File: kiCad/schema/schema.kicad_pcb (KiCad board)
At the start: 2 copper layers, 103.8 x 139.4 mm, 20 parts, among them J1 Conn_01x06_Pin, J11 Switch, J12 Conn_01x15_Pin, J13 Conn_01x15_Pin, J14 Conn_01x06_Pin, J3 M1 Right, J4 M2 Left, J5 Bat, J6 Buck, Q1 Q_Photo_NPN, Q2 Q_Photo_NPN, Q3 Q_Photo_NPN, Q4 Q_Photo_NPN

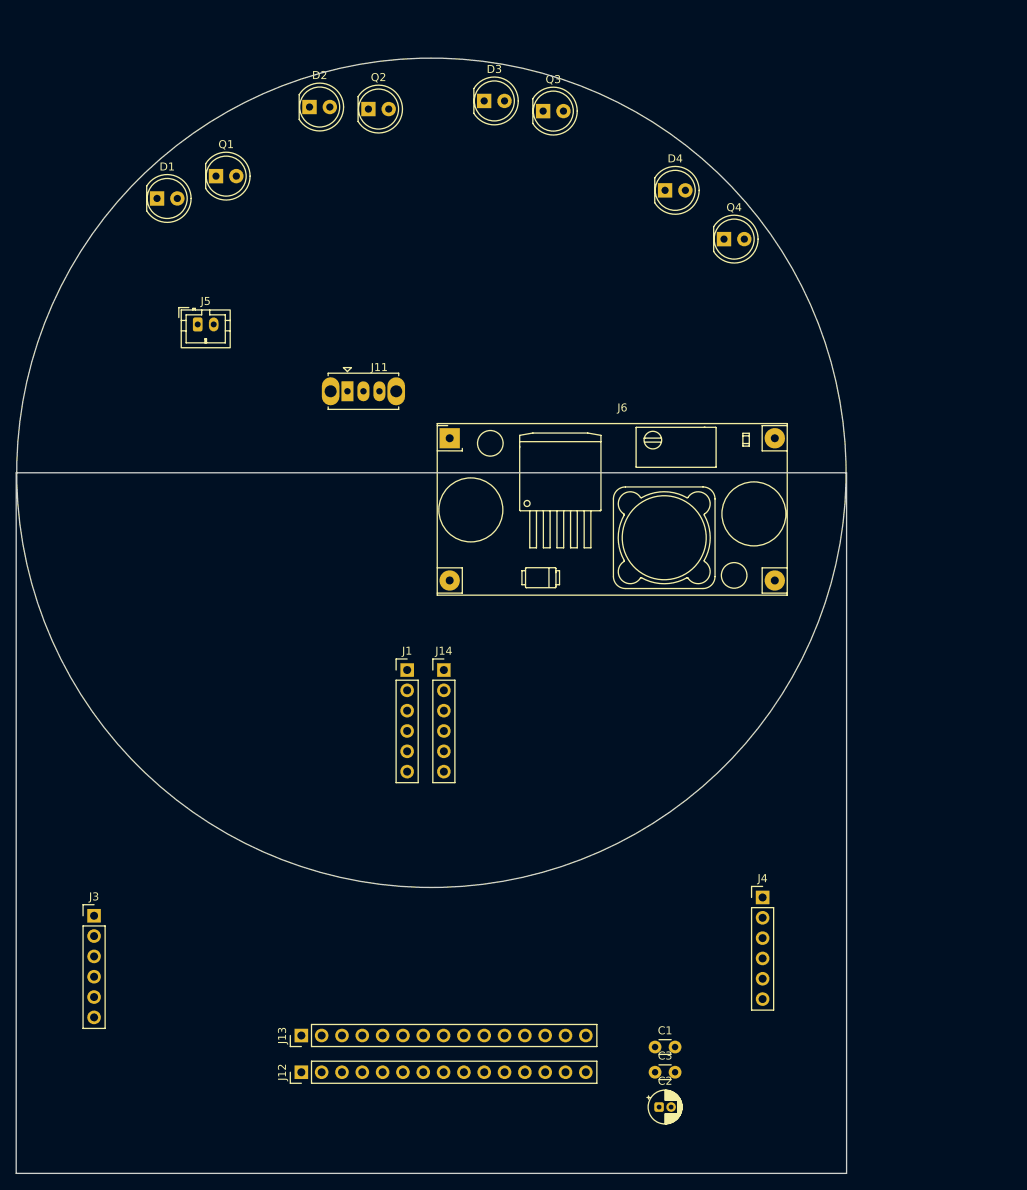
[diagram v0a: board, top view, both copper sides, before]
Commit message: Day 14 -- whole schematics done with footprints
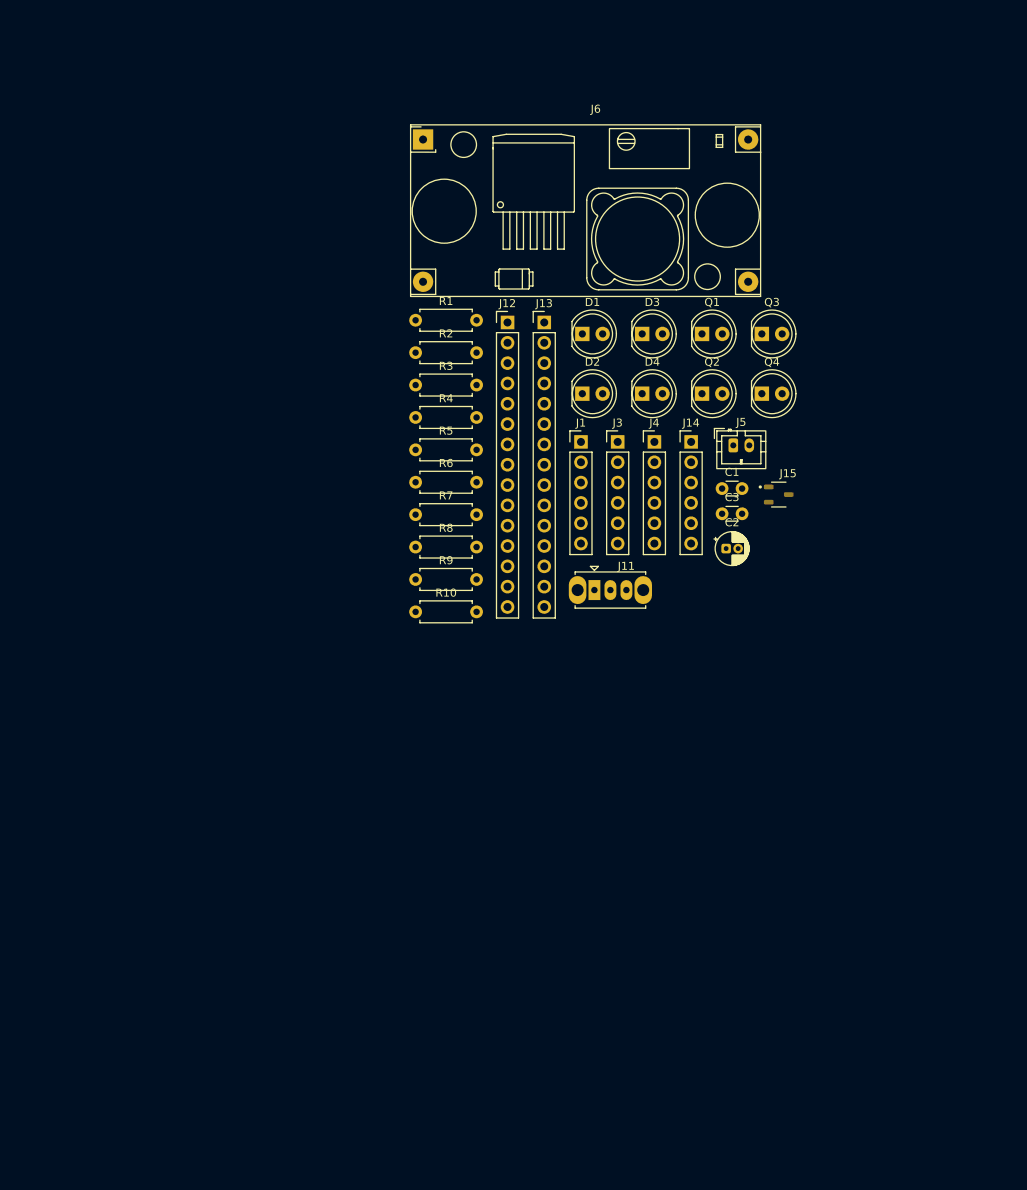
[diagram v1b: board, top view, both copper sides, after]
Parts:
- added J15: MOSFET, footprints:SOT95P280X125-3N, F.Cu at (118.4, 88.8)
- added R1: 120 ohm, Resistor_THT:R_Axial_DIN0207_L6.3mm_D2.5mm_P7.62mm_Horizontal, F.Cu at (73.0, 67.0)
- added R10: 10k ohm, Resistor_THT:R_Axial_DIN0207_L6.3mm_D2.5mm_P7.62mm_Horizontal, F.Cu at (73.0, 103.5)
- added R2: 120 ohm, Resistor_THT:R_Axial_DIN0207_L6.3mm_D2.5mm_P7.62mm_Horizontal, F.Cu at (73.0, 71.1)
- added R3: 120 ohm, Resistor_THT:R_Axial_DIN0207_L6.3mm_D2.5mm_P7.62mm_Horizontal, F.Cu at (73.0, 75.1)
- added R4: 120 ohm, Resistor_THT:R_Axial_DIN0207_L6.3mm_D2.5mm_P7.62mm_Horizontal, F.Cu at (73.0, 79.2)
- added R5: 100 ohm, Resistor_THT:R_Axial_DIN0207_L6.3mm_D2.5mm_P7.62mm_Horizontal, F.Cu at (73.0, 83.2)
- added R6: 100k ohm, Resistor_THT:R_Axial_DIN0207_L6.3mm_D2.5mm_P7.62mm_Horizontal, F.Cu at (73.0, 87.3)
- added R7: 10k ohm, Resistor_THT:R_Axial_DIN0207_L6.3mm_D2.5mm_P7.62mm_Horizontal, F.Cu at (73.0, 91.3)
- added R8: 10k ohm, Resistor_THT:R_Axial_DIN0207_L6.3mm_D2.5mm_P7.62mm_Horizontal, F.Cu at (73.0, 95.4)
- added R9: 10k ohm, Resistor_THT:R_Axial_DIN0207_L6.3mm_D2.5mm_P7.62mm_Horizontal, F.Cu at (73.0, 99.4)
- moved J12 97.2 mm to (84.4, 67.3), turned to 0 degrees
- moved J13 94.2 mm to (89.0, 67.3), turned to 0 degrees
- moved J3 88.3 mm to (98.2, 82.2)
- moved C1 70.3 mm to (111.3, 88.1)
- moved C2 70.3 mm to (111.8, 95.6)
- moved C3 70.3 mm to (111.3, 91.2)
- moved J5 68.6 mm to (112.7, 82.7)
- moved Q1 63.9 mm to (108.8, 68.7)
- moved J4 58.5 mm to (102.8, 82.2)
- moved D1 55.8 mm to (93.8, 68.7)
- moved Q2 54.8 mm to (108.8, 76.2)
- moved D2 49.5 mm to (93.8, 76.2)
- moved J14 42.1 mm to (107.4, 82.2)
- moved J11 39.6 mm to (95.3, 100.8)
- moved Q3 39.0 mm to (116.2, 68.7)
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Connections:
- J12 pad 12: unconnected-(J12-Pin_12-Pad12) -> /IR EM
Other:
- board outline removed

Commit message: Day 14 -- PCB layout
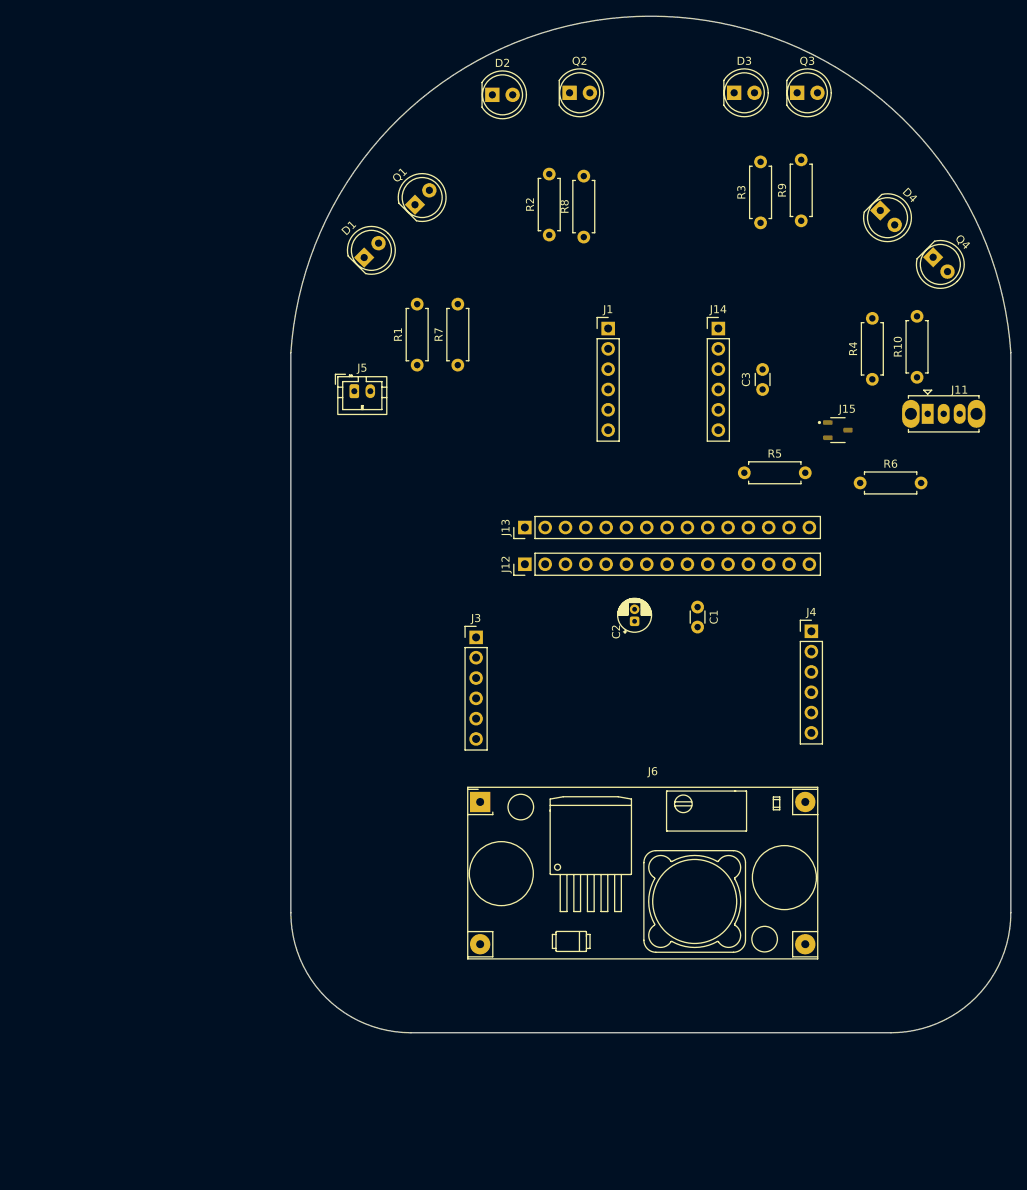
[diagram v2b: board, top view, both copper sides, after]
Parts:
- moved J6 83.1 mm to (81.0, 127.3)
- moved R10 69.2 mm to (135.6, 74.2), turned to 90 degrees
- moved R9 65.8 mm to (121.2, 54.6), turned to 90 degrees
- moved R4 57.3 mm to (130.0, 74.4), turned to 90 degrees
- moved R6 55.6 mm to (128.5, 87.4)
- moved J5 47.9 mm to (65.3, 75.9)
- moved R3 47.6 mm to (116.1, 54.9), turned to 90 degrees
- moved J11 47.1 mm to (137.0, 78.7)
- moved R8 44.1 mm to (94.0, 56.6), turned to 90 degrees
- moved R5 41.2 mm to (114.0, 86.1)
- moved Q2 41.1 mm to (92.2, 38.6)
- moved Q1 39.3 mm to (72.9, 52.6), turned to 45 degrees
- moved D2 39.0 mm to (82.5, 38.9)
- moved D4 37.6 mm to (131.0, 53.3), turned to -45 degrees
- moved D3 32.3 mm to (112.8, 38.6)
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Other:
- board outline added: 90 x 127.1 mm
